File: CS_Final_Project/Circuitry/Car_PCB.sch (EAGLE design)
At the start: 26 parts, among them SW1 KMR2, SW2 KMR2, U1 SPX3819, U2 DRV8830, X1 ESP-12, X2 22-23-2021, X3 22-23-2021

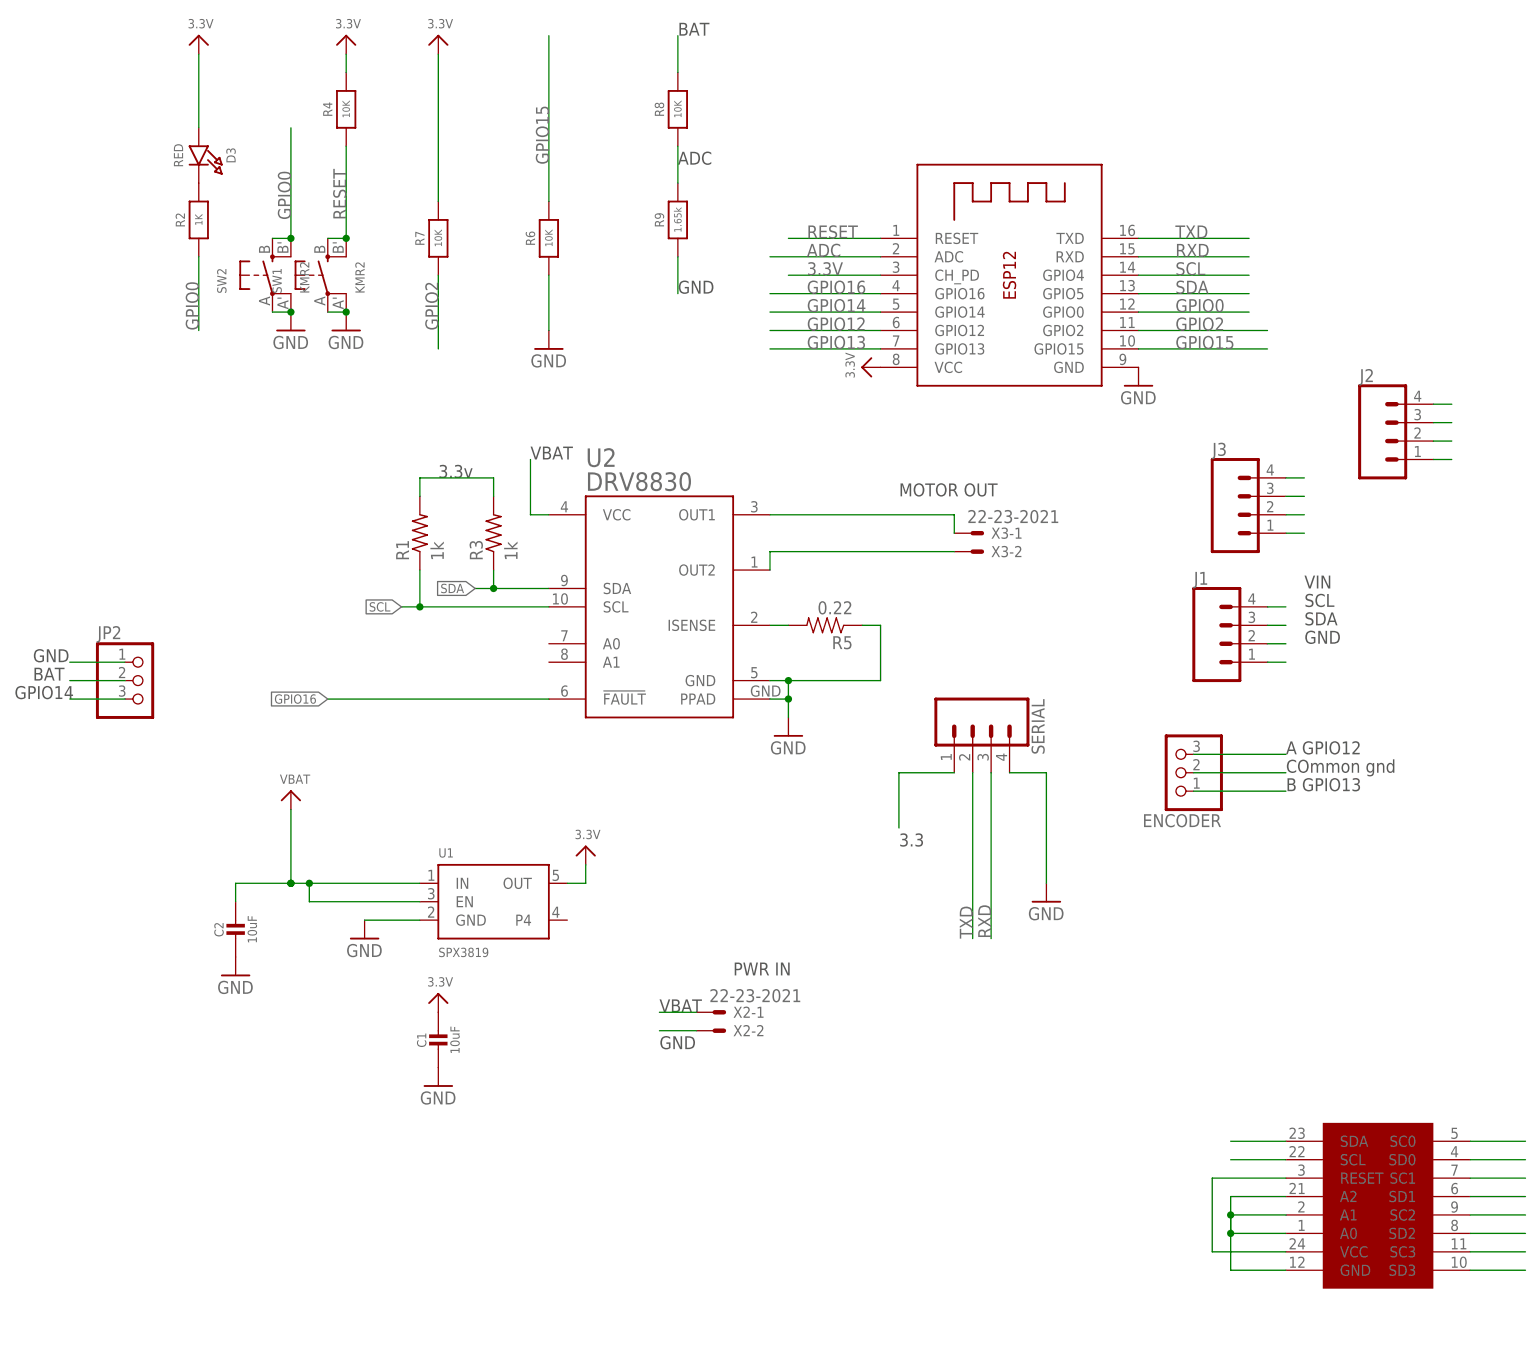
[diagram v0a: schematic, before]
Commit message: m
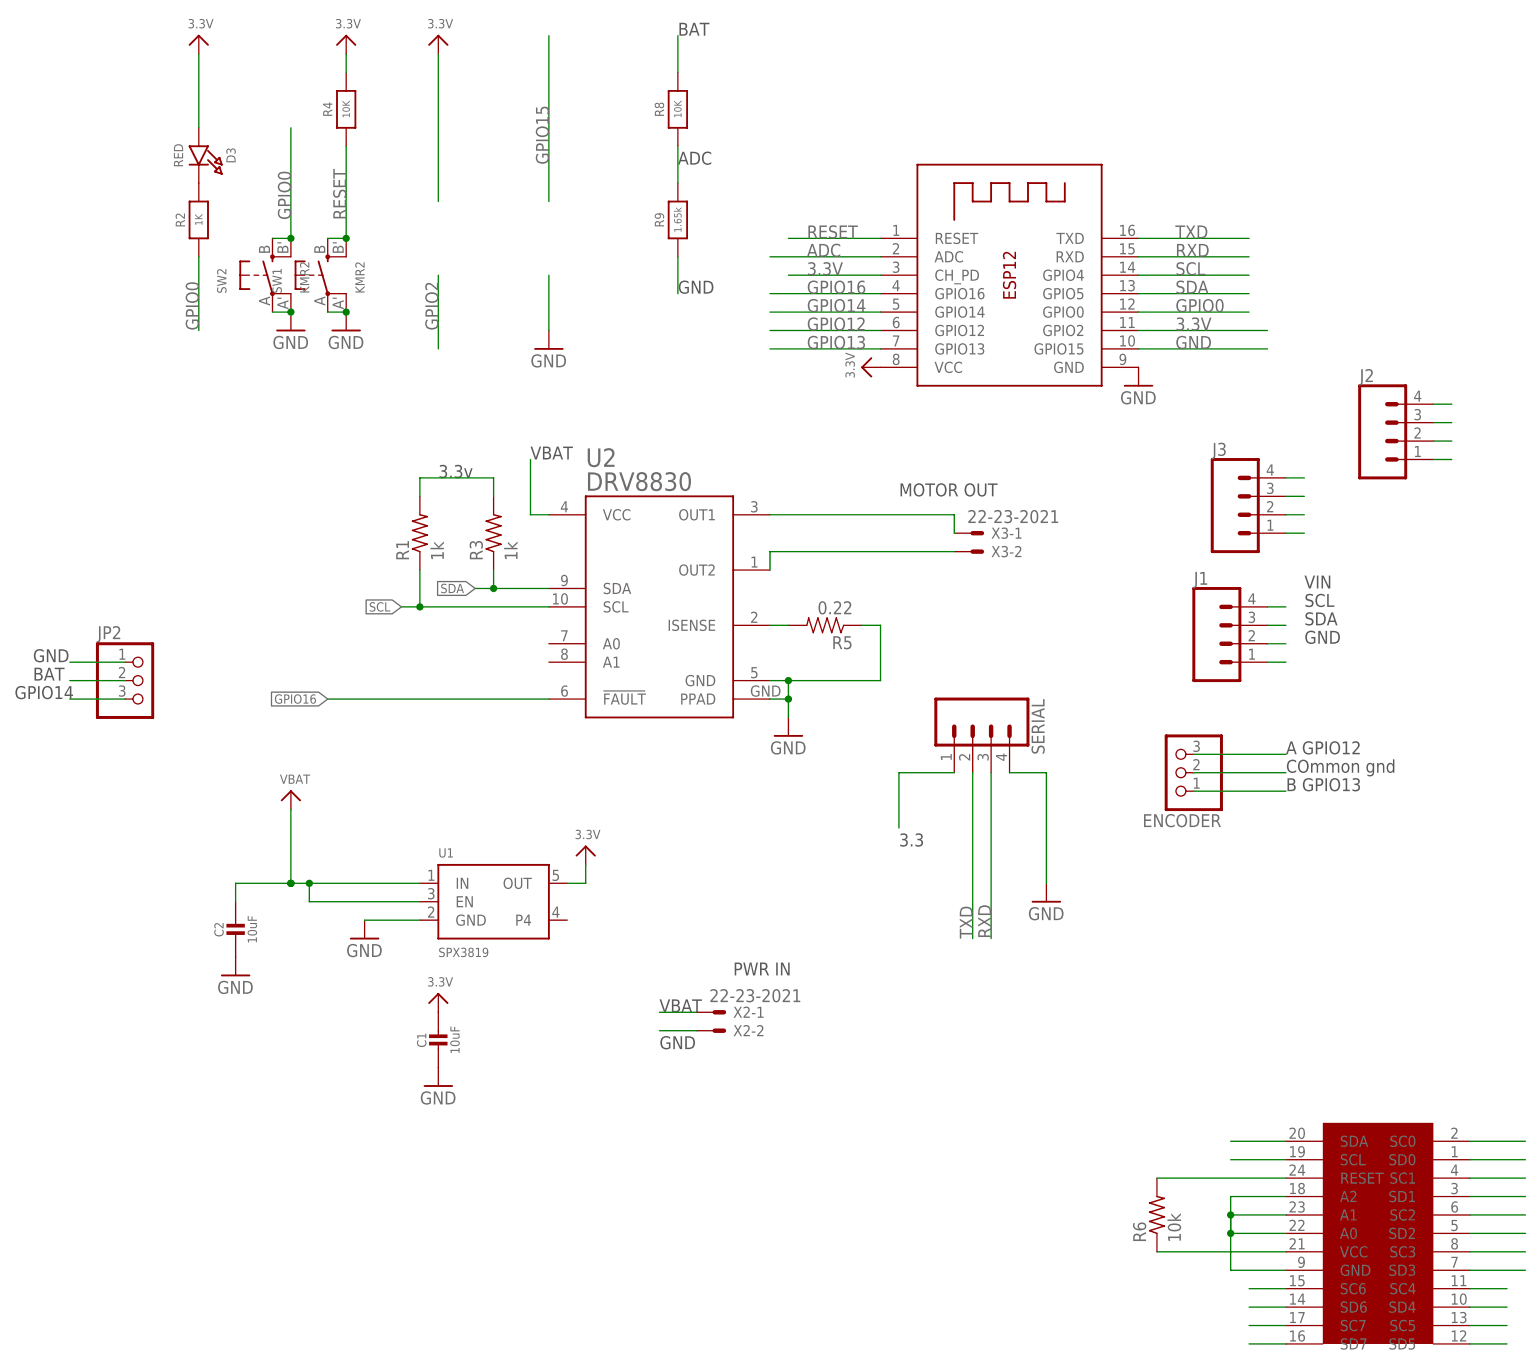
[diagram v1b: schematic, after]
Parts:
- removed R7: 10K, microbuilder:RESISTOR0805_NOOUTLINE
- R6: value 10K -> 10k; device microbuilder:RESISTOR0805_NOOUTLINE -> adafruit:R-US_M0805
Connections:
- removed net GPIO15: R6.2, X1.GPIO15
- removed net GPIO2: R7.1, X1.GPIO2
- new net N$5: R6.2, U$1.RESET
- new net SC4: U$1.SC4
- new net SC5: J2.2, U$1.SC5
- new net SC6: J1.2, U$1.SC6
- new net SC7: U$1.SC7
- new net SD4: U$1.SD4
- new net SD5: J2.3, U$1.SD5
- new net SD6: J1.3, U$1.SD6
- new net SD7: U$1.SD7
- net 3.3V: now also R6.1, X1.GPIO2; no longer R7.2, U$1.RESET
- net GND: now also X1.GPIO15; no longer R6.1
- net SC0: no longer J1.3
- net SC1: no longer J2.3
- net SC3: now also J3.2; no longer J3.3
- net SD0: no longer J1.2
- net SD1: no longer J2.2
- net SD3: now also J3.3; no longer J3.2
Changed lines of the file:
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@@
 <part name="R4" library="microbuilder" deviceset="RESISTOR" device="0805_NOOUTLINE" value="10K"/>
 <part name="U$4" library="microbuilder" deviceset="3.3V" device=""/>
-<part name="R6" library="microbuilder" deviceset="RESISTOR" device="0805_NOOUTLINE" value="10K"/>
 <part name="GND1" library="supply1" deviceset="GND" device=""/>
 <part name="U$11" library="microbuilder" deviceset="VBAT" device=""/>
-<part name="R7" library="microbuilder" deviceset="RESISTOR" device="0805_NOOUTLINE" value="10K"/>
 <part name="U$5" library="microbuilder" deviceset="3.3V" device=""/>
 <part name="SW1" library="microbuilder" deviceset="SWITCH_TACT_SMT" device="4.6X2.8" value="KMR2"/>
@@
 <part name="J3" library="SparkFun-Connectors" deviceset="CONN_04" device=""/>
 <part name="U$1" library="si70xx-10" deviceset="TCA9548A" device=""/>
+<part name="R6" library="adafruit" deviceset="R-US_" device="M0805" value="10k"/>
 </parts>
 <sheets>
@@
 <instance part="R4" gate="G$1" x="-7.62" y="144.78" rot="R90"/>
 <instance part="U$4" gate="G$1" x="-7.62" y="154.94"/>
-<instance part="R6" gate="G$1" x="20.32" y="127" rot="R90"/>
 <instance part="GND1" gate="1" x="20.32" y="111.76"/>
 <instance part="U$11" gate="G$1" x="-15.24" y="50.8"/>
-<instance part="R7" gate="G$1" x="5.08" y="127" rot="R90"/>
 <instance part="U$5" gate="G$1" x="5.08" y="154.94"/>
 <instance part="SW1" gate="G$1" x="-10.16" y="121.92" rot="R90"/>
@@
 <instance part="J3" gate="G$1" x="116.84" y="88.9"/>
 <instance part="U$1" gate="G$1" x="127" y="-5.08"/>
+<instance part="R6" gate="G$1" x="104.14" y="-7.62" rot="R90"/>
 </instances>
 <busses>
@@
 </segment>
 <segment>
-<pinref part="R6" gate="G$1" pin="1"/>
 <pinref part="GND1" gate="1" pin="GND"/>
 <wire x1="20.32" y1="114.3" x2="20.32" y2="121.92" width="0.1524" layer="91"/>
@@
 <wire x1="142.24" y1="96.52" x2="144.78" y2="96.52" width="0.1524" layer="91"/>
 </segment>
+<segment>
+<pinref part="X1" gate="G$1" pin="GPIO15"/>
+<wire x1="101.6" y1="111.76" x2="119.38" y2="111.76" width="0.1524" layer="91"/>
+<label x="106.68" y="111.76" size="1.778" layer="95"/>
+</segment>
 </net>
 <net name="3.3V" class="0">
@@
 </segment>
 <segment>
-<pinref part="R7" gate="G$1" pin="2"/>
 <pinref part="U$5" gate="G$1" pin="3.3V"/>
 <wire x1="5.08" y1="132.08" x2="5.08" y2="152.4" width="0.1524" layer="91"/>
@@
 </segment>
 <segment>
-<pinref part="U$1" gate="G$1" pin="VCC"/>
-<wire x1="121.92" y1="-12.7" x2="111.76" y2="-12.7" width="0.1524" layer="91"/>
-<pinref part="U$1" gate="G$1" pin="RESET"/>
-<wire x1="121.92" y1="-2.54" x2="111.76" y2="-2.54" width="0.1524" layer="91"/>
-<wire x1="111.76" y1="-2.54" x2="111.76" y2="-12.7" width="0.1524" layer="91"/>
-</segment>
-<segment>
 <pinref part="J3" gate="G$1" pin="4"/>
 <wire x1="121.92" y1="93.98" x2="124.46" y2="93.98" width="0.1524" layer="91"/>
@@
 <pinref part="J2" gate="G$1" pin="4"/>
 <wire x1="142.24" y1="104.14" x2="144.78" y2="104.14" width="0.1524" layer="91"/>
+</segment>
+<segment>
+<pinref part="X1" gate="G$1" pin="GPIO2"/>
+<wire x1="119.38" y1="114.3" x2="101.6" y2="114.3" width="0.1524" layer="91"/>
+<label x="106.68" y="114.3" size="1.778" layer="95"/>
+</segment>
+<segment>
+<pinref part="U$1" gate="G$1" pin="VCC"/>
+<wire x1="121.92" y1="-12.7" x2="104.14" y2="-12.7" width="0.1524" layer="91"/>
+<pinref part="R6" gate="G$1" pin="1"/>
 </segment>
 </net>
@@
 <net name="GPIO15" class="0">
 <segment>
-<pinref part="X1" gate="G$1" pin="GPIO15"/>
-<wire x1="101.6" y1="111.76" x2="119.38" y2="111.76" width="0.1524" layer="91"/>
-<label x="106.68" y="111.76" size="1.778" layer="95"/>
-</segment>
-<segment>
-<pinref part="R6" gate="G$1" pin="2"/>
 <wire x1="20.32" y1="132.08" x2="20.32" y2="154.94" width="0.1524" layer="91"/>
 <label x="20.32" y="137.16" size="1.778" layer="95" rot="R90"/>
@@
 <net name="GPIO2" class="0">
 <segment>
-<pinref part="X1" gate="G$1" pin="GPIO2"/>
-<wire x1="119.38" y1="114.3" x2="101.6" y2="114.3" width="0.1524" layer="91"/>
-<label x="106.68" y="114.3" size="1.778" layer="95"/>
-</segment>
-<segment>
-<pinref part="R7" gate="G$1" pin="1"/>
 <wire x1="5.08" y1="121.92" x2="5.08" y2="111.76" width="0.1524" layer="91"/>
 <label x="5.08" y="114.3" size="1.778" layer="95" rot="R90"/>
@@
 <wire x1="147.32" y1="2.54" x2="154.94" y2="2.54" width="0.1524" layer="91"/>
 </segment>
+</net>
+<net name="SD0" class="0">
+<segment>
+<pinref part="U$1" gate="G$1" pin="SD0"/>
+<wire x1="147.32" y1="0" x2="154.94" y2="0" width="0.1524" layer="91"/>
+</segment>
+</net>
+<net name="SC1" class="0">
+<segment>
+<pinref part="U$1" gate="G$1" pin="SC1"/>
+<wire x1="147.32" y1="-2.54" x2="154.94" y2="-2.54" width="0.1524" layer="91"/>
+</segment>
+</net>
+<net name="SD1" class="0">
+<segment>
+<pinref part="U$1" gate="G$1" pin="SD1"/>
+<wire x1="147.32" y1="-5.08" x2="154.94" y2="-5.08" width="0.1524" layer="91"/>
+</segment>
+</net>
+<net name="SC2" class="0">
+<segment>
+<pinref part="U$1" gate="G$1" pin="SC2"/>
+<wire x1="147.32" y1="-7.62" x2="154.94" y2="-7.62" width="0.1524" layer="91"/>
+</segment>
+</net>
+<net name="SD2" class="0">
+<segment>
+<pinref part="U$1" gate="G$1" pin="SD2"/>
+<wire x1="147.32" y1="-10.16" x2="154.94" y2="-10.16" width="0.1524" layer="91"/>
+</segment>
+</net>
+<net name="SC3" class="0">
+<segment>
+<pinref part="U$1" gate="G$1" pin="SC3"/>
+<wire x1="147.32" y1="-12.7" x2="154.94" y2="-12.7" width="0.1524" layer="91"/>
+</segment>
+<segment>
+<pinref part="J3" gate="G$1" pin="2"/>
+<wire x1="121.92" y1="88.9" x2="124.46" y2="88.9" width="0.1524" layer="91"/>
+</segment>
+</net>
+<net name="SD3" class="0">
+<segment>
+<pinref part="U$1" gate="G$1" pin="SD3"/>
+<wire x1="147.32" y1="-15.24" x2="154.94" y2="-15.24" width="0.1524" layer="91"/>
+</segment>
+<segment>
+<pinref part="J3" gate="G$1" pin="3"/>
+<wire x1="121.92" y1="91.44" x2="124.46" y2="91.44" width="0.1524" layer="91"/>
+</segment>
+</net>
+<net name="SC6" class="0">
+<segment>
+<pinref part="U$1" gate="G$1" pin="SC6"/>
+<wire x1="121.92" y1="-17.78" x2="116.84" y2="-17.78" width="0.1524" layer="91"/>
+</segment>
+<segment>
+<pinref part="J1" gate="G$1" pin="2"/>
+<wire x1="119.38" y1="71.12" x2="121.92" y2="71.12" width="0.1524" layer="91"/>
+</segment>
+</net>
+<net name="SD6" class="0">
+<segment>
+<pinref part="U$1" gate="G$1" pin="SD6"/>
+<wire x1="121.92" y1="-20.32" x2="116.84" y2="-20.32" width="0.1524" layer="91"/>
+</segment>
 <segment>
 <pinref part="J1" gate="G$1" pin="3"/>
@@
 </segment>
 </net>
-<net name="SD0" class="0">
-<segment>
-<pinref part="U$1" gate="G$1" pin="SD0"/>
-<wire x1="147.32" y1="0" x2="154.94" y2="0" width="0.1524" layer="91"/>
-</segment>
-<segment>
-<pinref part="J1" gate="G$1" pin="2"/>
-<wire x1="119.38" y1="71.12" x2="121.92" y2="71.12" width="0.1524" layer="91"/>
-</segment>
-</net>
-<net name="SC1" class="0">
-<segment>
-<pinref part="U$1" gate="G$1" pin="SC1"/>
-<wire x1="147.32" y1="-2.54" x2="154.94" y2="-2.54" width="0.1524" layer="91"/>
+<net name="SC7" class="0">
+<segment>
+<pinref part="U$1" gate="G$1" pin="SC7"/>
+<wire x1="121.92" y1="-22.86" x2="116.84" y2="-22.86" width="0.1524" layer="91"/>
+</segment>
+</net>
+<net name="SD7" class="0">
+<segment>
+<pinref part="U$1" gate="G$1" pin="SD7"/>
+<wire x1="121.92" y1="-25.4" x2="116.84" y2="-25.4" width="0.1524" layer="91"/>
+</segment>
+</net>
+<net name="SC4" class="0">
+<segment>
+<pinref part="U$1" gate="G$1" pin="SC4"/>
+<wire x1="147.32" y1="-17.78" x2="152.4" y2="-17.78" width="0.1524" layer="91"/>
+</segment>
+</net>
+<net name="SD4" class="0">
+<segment>
+<pinref part="U$1" gate="G$1" pin="SD4"/>
+<wire x1="147.32" y1="-20.32" x2="152.4" y2="-20.32" width="0.1524" layer="91"/>
+</segment>
+</net>
+<net name="SC5" class="0">
+<segment>
+<pinref part="U$1" gate="G$1" pin="SC5"/>
+<wire x1="147.32" y1="-22.86" x2="152.4" y2="-22.86" width="0.1524" layer="91"/>
+</segment>
+<segment>
+<pinref part="J2" gate="G$1" pin="2"/>
+<wire x1="142.24" y1="99.06" x2="144.78" y2="99.06" width="0.1524" layer="91"/>
+</segment>
+</net>
+<net name="SD5" class="0">
+<segment>
+<pinref part="U$1" gate="G$1" pin="SD5"/>
+<wire x1="147.32" y1="-25.4" x2="152.4" y2="-25.4" width="0.1524" layer="91"/>
 </segment>
 <segment>
@@
 </segment>
 </net>
-<net name="SD1" class="0">
-<segment>
-<pinref part="U$1" gate="G$1" pin="SD1"/>
-<wire x1="147.32" y1="-5.08" x2="154.94" y2="-5.08" width="0.1524" layer="91"/>
-</segment>
-<segment>
-<pinref part="J2" gate="G$1" pin="2"/>
-<wire x1="142.24" y1="99.06" x2="144.78" y2="99.06" width="0.1524" layer="91"/>
-</segment>
-</net>
-<net name="SC2" class="0">
-<segment>
-<pinref part="U$1" gate="G$1" pin="SC2"/>
-<wire x1="147.32" y1="-7.62" x2="154.94" y2="-7.62" width="0.1524" layer="91"/>
-</segment>
-</net>
-<net name="SD2" class="0">
-<segment>
-<pinref part="U$1" gate="G$1" pin="SD2"/>
-<wire x1="147.32" y1="-10.16" x2="154.94" y2="-10.16" width="0.1524" layer="91"/>
-</segment>
-</net>
-<net name="SC3" class="0">
-<segment>
-<pinref part="U$1" gate="G$1" pin="SC3"/>
-<wire x1="147.32" y1="-12.7" x2="154.94" y2="-12.7" width="0.1524" layer="91"/>
-</segment>
-<segment>
-<pinref part="J3" gate="G$1" pin="3"/>
-<wire x1="121.92" y1="91.44" x2="124.46" y2="91.44" width="0.1524" layer="91"/>
-</segment>
-</net>
-<net name="SD3" class="0">
-<segment>
-<pinref part="U$1" gate="G$1" pin="SD3"/>
-<wire x1="147.32" y1="-15.24" x2="154.94" y2="-15.24" width="0.1524" layer="91"/>
-</segment>
-<segment>
-<pinref part="J3" gate="G$1" pin="2"/>
-<wire x1="121.92" y1="88.9" x2="124.46" y2="88.9" width="0.1524" layer="91"/>
-</segment>
-</net>
+<net name="N$5" class="0">
+<segment>
+<pinref part="U$1" gate="G$1" pin="RESET"/>
+<wire x1="121.92" y1="-2.54" x2="104.14" y2="-2.54" width="0.1524" layer="91"/>
+<pinref part="R6" gate="G$1" pin="2"/>
+</segment>
+</net>
